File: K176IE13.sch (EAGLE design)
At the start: 106 parts, among them J1 0R-JUMPB

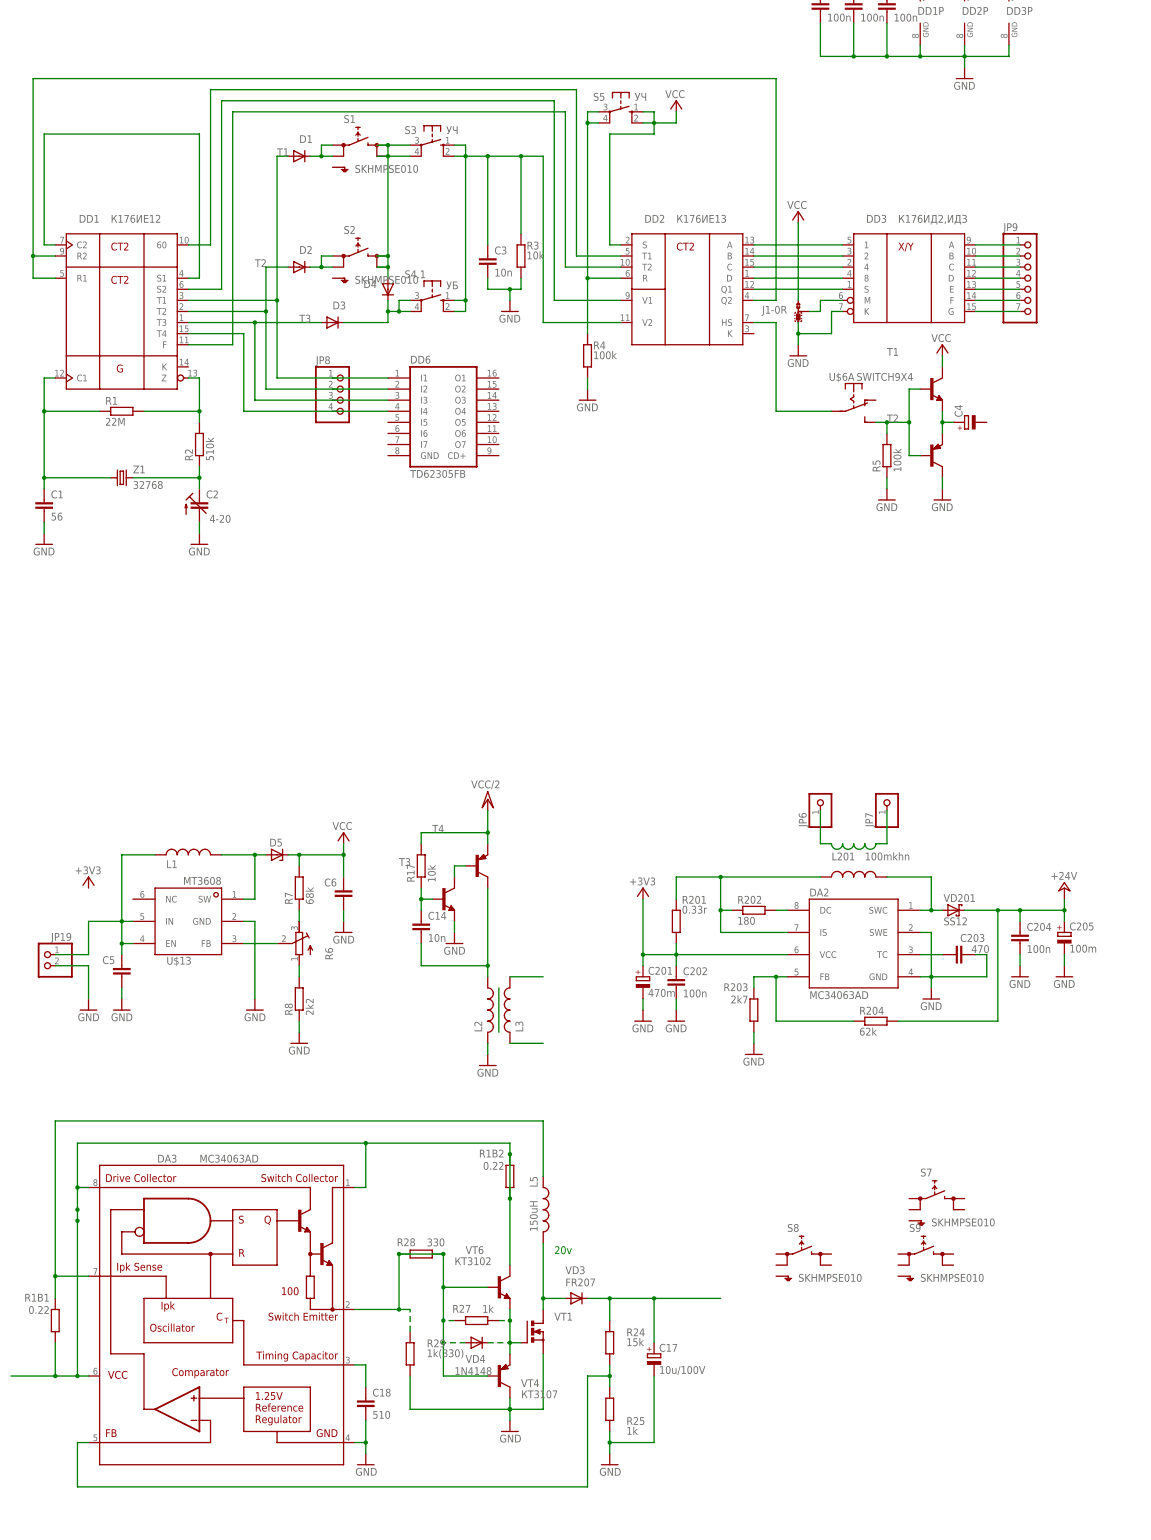
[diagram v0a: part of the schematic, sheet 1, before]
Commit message: .
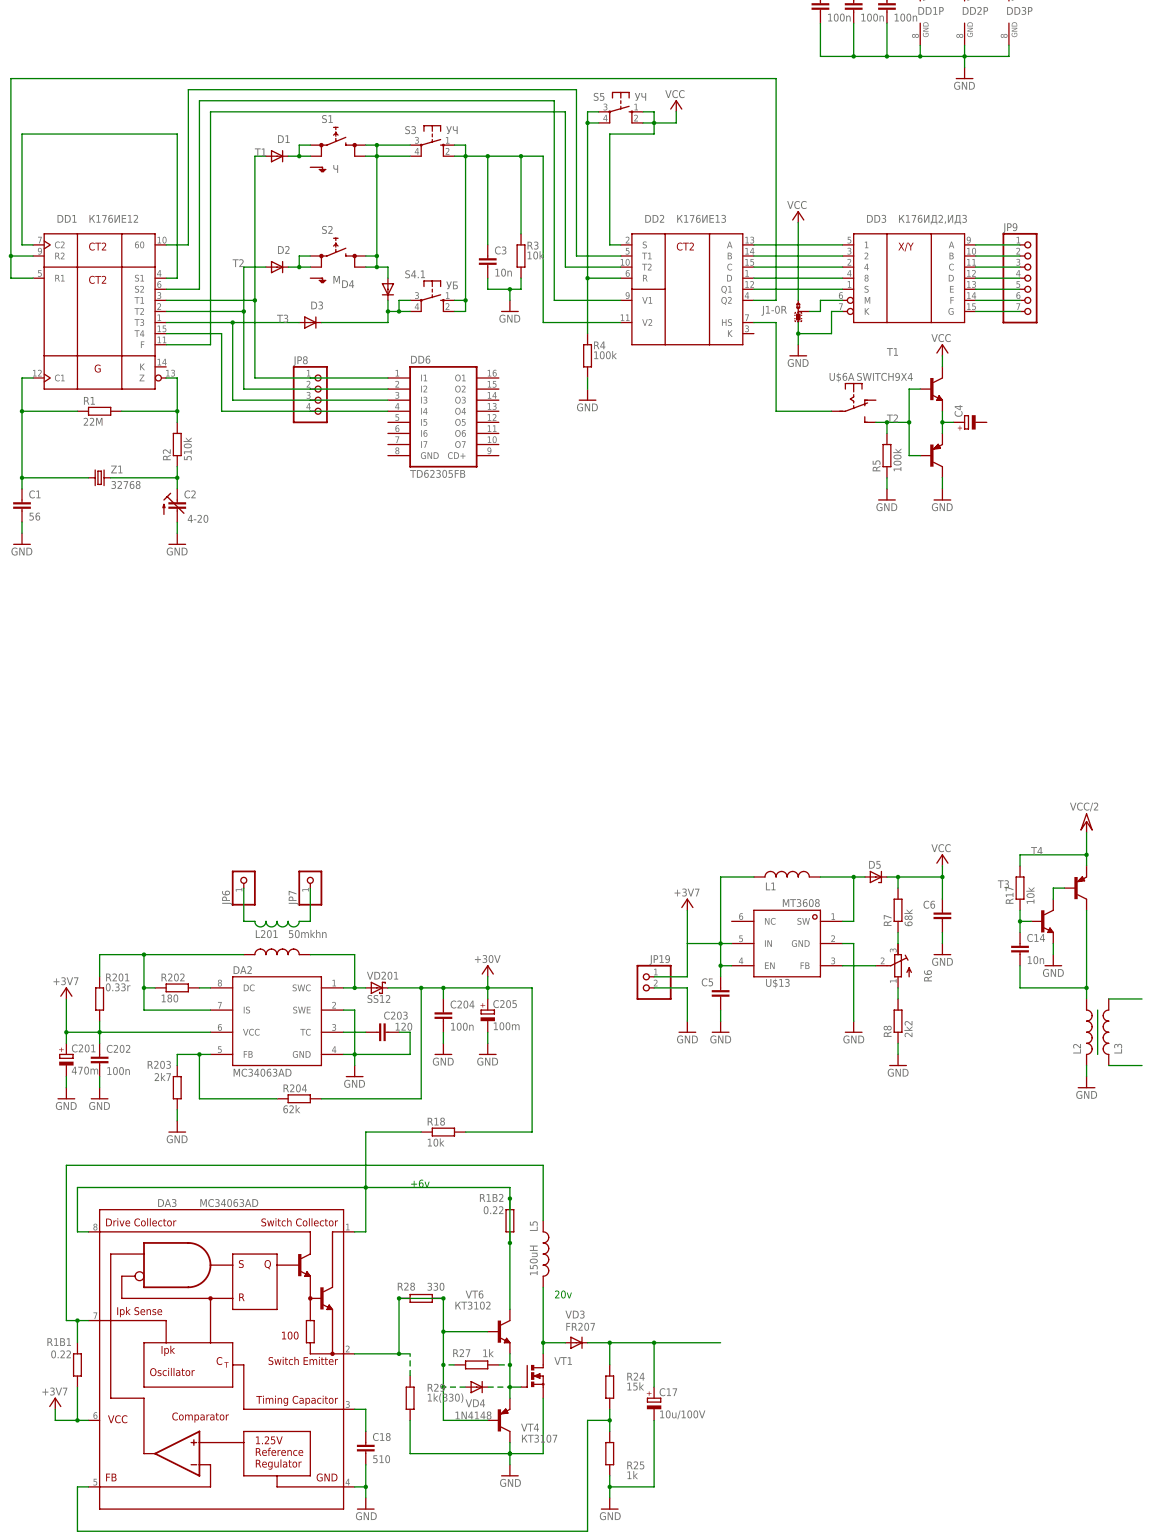
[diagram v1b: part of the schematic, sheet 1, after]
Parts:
- removed S7, S8, S9: SKHMPSE010, switch:SKHMPSE010
- added R18: 10k, rcl:R-EU_M0805
- C203: value 470 -> 120
- L201: value 100mkhn -> 50mkhn
- S1: value SKHMPSE010 -> Ч
- S2: value SKHMPSE010 -> М
- V3: value ИВ-6 -> ИВ-3А
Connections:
- removed net +24V: C204.1, C205.+, R204.2, VD201.C
- removed net N$28: C5.1, JP19.1, L1.2, U$13.EN, U$13.IN
- removed net N$96: DA3.DC, DA3.SWC, DA3.VCC, R1B1.1, R1B2.1, R1B2.2, VT6.C
- new net +30V: C204.1, C205.+, R18.2, R204.2, VD201.C
- new net N$26: DA3.DC, DA3.SWC, R18.1, R1B2.1, R1B2.2, VT6.C
- net +3V3: now also C5.1, DA3.VCC, JP19.1, L1.2, R1B1.1, U$13.EN, U$13.IN
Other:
- note added: "+6v"
- moved on the sheet: C1, C14, C17, C18, C2, C201, C202, C203, C204, C205, C5, C6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
